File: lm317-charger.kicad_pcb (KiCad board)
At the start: 2 copper layers, 12 parts, among them J1 Conn_01x02_Socket, J2 Conn_01x02_Socket, SW1 SW_SPDT, U1 LM317_TO-220, U2 LM317_TO-220

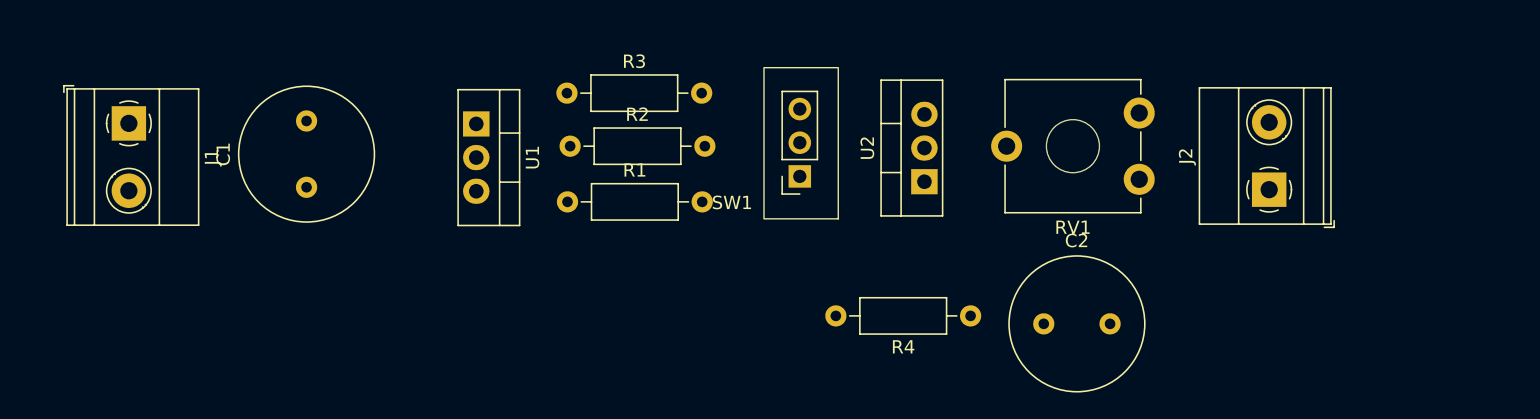
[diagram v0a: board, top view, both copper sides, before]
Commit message: update
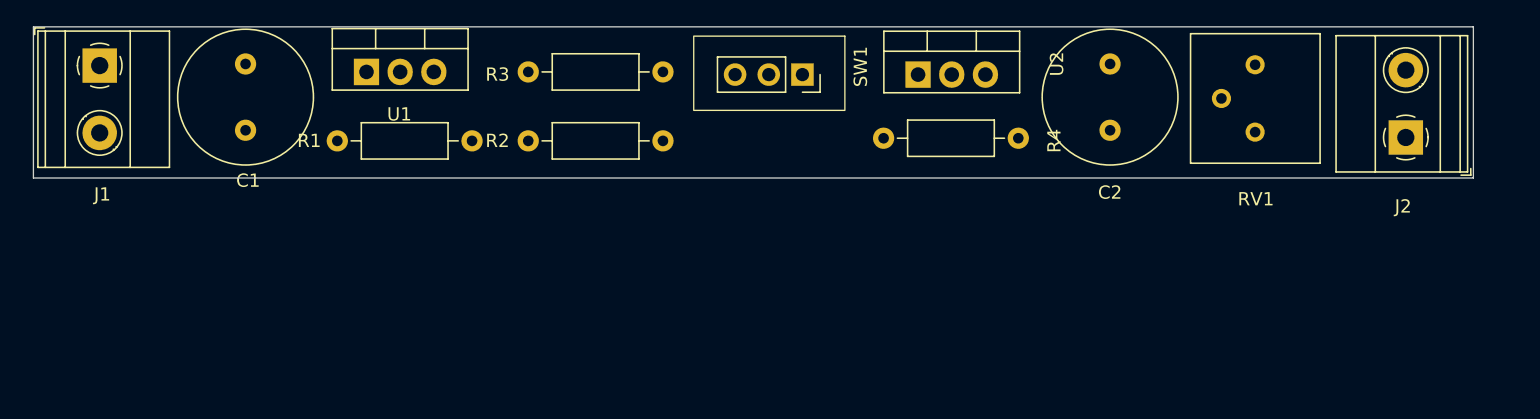
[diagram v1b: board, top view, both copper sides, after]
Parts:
- RV1: footprint Potentiometer_THT:Potentiometer_ACP_CA9-V10_Vertical_Hole -> Potentiometer_THT:Potentiometer_Bourns_3386P_Vertical
- moved R1 18.0 mm to (55.9, 39.6)
- moved C2 15.4 mm to (114.2, 38.8), turned to 90 degrees
- moved R4 14.9 mm to (97.1, 39.4), turned to 0 degrees
- moved J2 11.0 mm to (136.5, 39.3)
- moved RV1 9.47 mm to (125.1, 33.9)
- moved U1 9.16 mm to (58.1, 34.4), turned to 0 degrees
- moved U2 8.09 mm to (99.7, 34.6), turned to 0 degrees
- moved SW1 7.68 mm to (91.0, 34.6), turned to -90 degrees
- moved C1 6.30 mm to (49.0, 38.8)
- moved J1 4.88 mm to (38.0, 33.9)
- moved R3 3.33 mm to (70.3, 34.4)
- moved R2 3.19 mm to (70.3, 39.6)
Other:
- board outline added: 108.6 x 11.4 mm

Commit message: update
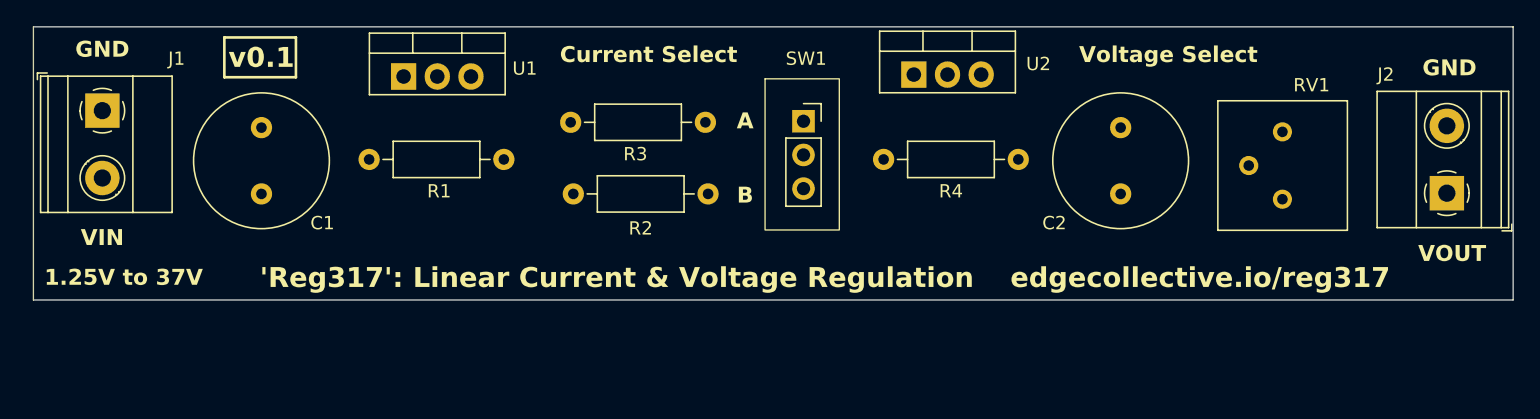
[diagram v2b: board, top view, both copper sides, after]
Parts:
- moved RV1 5.46 mm to (127.2, 38.9)
- moved R2 5.25 mm to (73.7, 43.6)
- moved J2 5.22 mm to (139.6, 43.5)
- moved R3 4.97 mm to (73.5, 38.2)
- moved C1 4.95 mm to (50.2, 43.6)
- moved C2 4.87 mm to (115.0, 43.6)
- moved SW1 3.52 mm to (91.1, 38.1), turned to 0 degrees
- moved J1 3.41 mm to (38.2, 37.3)
- moved U1 2.82 mm to (60.9, 34.7)
- moved R1 2.78 mm to (58.3, 41.0)
- moved R4 1.60 mm to (97.1, 41.0)
- moved U2 0.32 mm to (99.4, 34.6)
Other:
- board size 108.6 x 11.4 mm -> 111.6 x 20.6 mm
- board text added: "'Reg317': Linear Current & Voltage Regulation"
- board text added: "1.25V to 37V"
- board text added: "A"
- board text added: "B"
- board text added: "Current Select"
- board text added: "GND"
- board text added: "VIN"
- board text added: "VOUT"
- board text added: "Voltage Select"
- board text added: "edgecollective.io/reg317"
- board text added: "v0.1"
